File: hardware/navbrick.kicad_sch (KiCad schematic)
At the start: 28 parts, among them J50 Conn_01x06_Pin, J51 Conn_01x06_Pin, SW50 PTS645SK50SMTR92, SW51 PTS645SK50SMTR92, U6 AVR128DA32x-xRXB, U7 FM25L16B

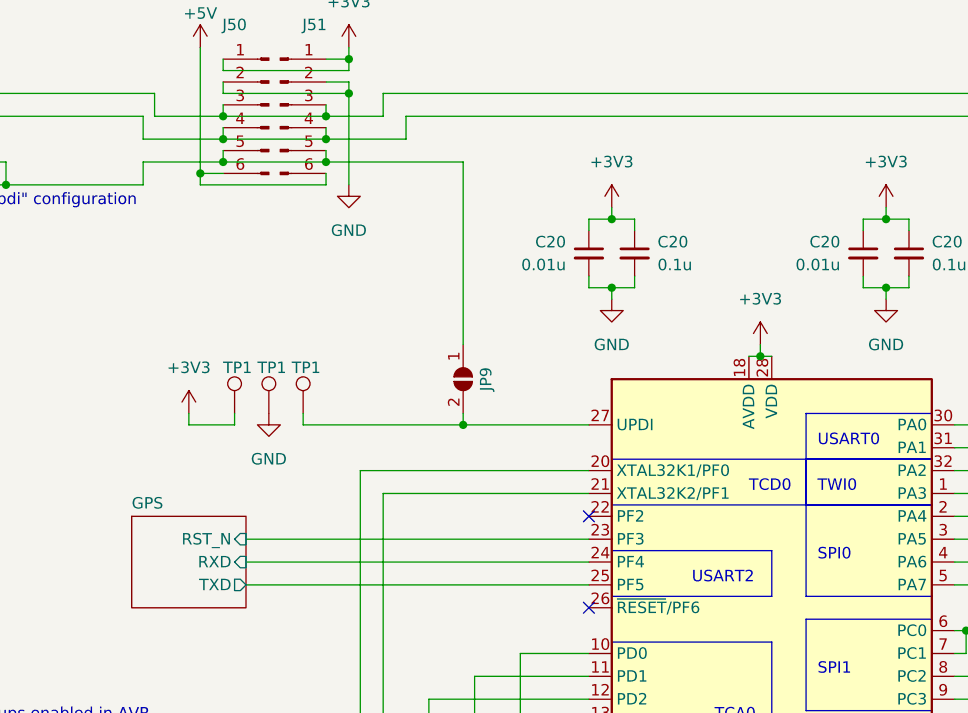
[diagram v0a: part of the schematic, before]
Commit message: Rev B hardware update
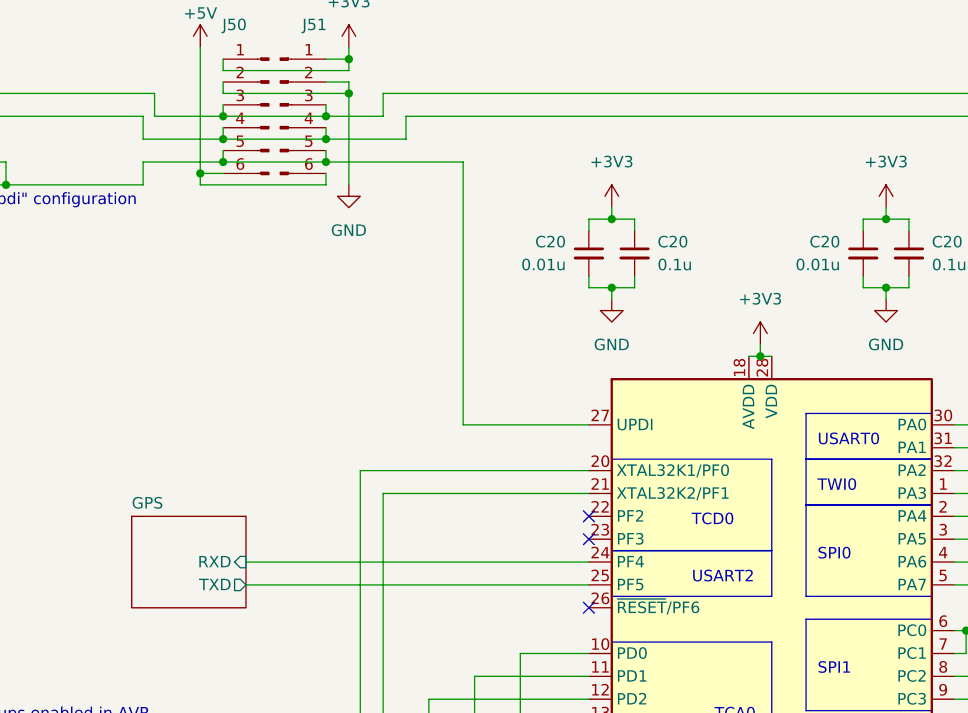
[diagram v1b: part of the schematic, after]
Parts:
- removed JP9: SolderJumper_2_Open, Jumper:SolderJumper-2_P1.3mm_Open_Pad1.0x1.5mm, symbol 0-passives:SolderJumper_2
- removed TP1 (x3): TestPoint, TestPoint:TestPoint_Pad_D2.0mm, symbol Connector:TestPoint
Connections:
- net USB/RxD_1: now also U6.27 (UPDI)
- net GPS/RST_N: no longer names the net of U6.23 (PF3)
- no-connect marks 2 -> 3
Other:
- sheet GPS ports: added none; removed RST_N
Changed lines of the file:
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@@
   (junction (at 53.34 36.83) (diameter 0) (color 0 0 0 0)
-  )
-  (junction (at 104.14 63.5) (diameter 0) (color 0 0 0 0)
   )
   (junction (at 151.13 40.64) (diameter 0) (color 0 0 0 0)
@@
   (no_connect (at 118.11 83.82))
   (no_connect (at 118.11 73.66))
+  (no_connect (at 118.11 76.2))
   (wire (pts (xy 53.34 36.83) (xy 68.58 36.83))
     (stroke (width 0) (type default))
@@
     (stroke (width 0) (type default))
   )
-  (wire (pts (xy 73.66 62.23) (xy 73.66 63.5))
-    (stroke (width 0) (type default))
-  )
   (wire (pts (xy 160.02 86.36) (xy 181.61 86.36))
     (stroke (width 0) (type default))
@@
     (stroke (width 0) (type default))
   )
-  (wire (pts (xy 86.36 62.23) (xy 86.36 63.5))
-    (stroke (width 0) (type default))
-  )
   (wire (pts (xy 92.71 146.05) (xy 92.71 68.58))
     (stroke (width 0) (type default))
@@
     (stroke (width 0) (type default))
   )
-  (wire (pts (xy 104.14 34.29) (xy 104.14 54.61))
+  (wire (pts (xy 104.14 34.29) (xy 104.14 63.5))
     (stroke (width 0) (type default))
   )
@@
     (stroke (width 0) (type default))
   )
-  (wire (pts (xy 104.14 62.23) (xy 104.14 63.5))
-    (stroke (width 0) (type default))
-  )
-  (wire (pts (xy 78.74 63.5) (xy 78.74 62.23))
-    (stroke (width 0) (type default))
-  )
   (wire (pts (xy 53.34 34.29) (xy 52.07 34.29))
     (stroke (width 0) (type default))
@@
     (stroke (width 0) (type default))
   )
-  (wire (pts (xy 86.36 63.5) (xy 104.14 63.5))
-    (stroke (width 0) (type default))
-  )
   (wire (pts (xy 88.9 31.75) (xy 88.9 30.48))
     (stroke (width 0) (type default))
@@
     (stroke (width 0) (type default))
   )
-  (wire (pts (xy 80.01 76.2) (xy 118.11 76.2))
-    (stroke (width 0) (type default))
-  )
   (wire (pts (xy 44.45 113.03) (xy 44.45 115.57))
     (stroke (width 0) (type default))
@@
     (stroke (width 0) (type default))
   )
-  (wire (pts (xy 73.66 63.5) (xy 78.74 63.5))
-    (stroke (width 0) (type default))
-  )
   (rectangle (start 142.24 85.09) (end 156.21 95.25)
     (stroke (width 0) (type default))
     (fill (type none))
   )
-  (rectangle (start 120.65 67.31) (end 142.24 72.39)
+  (rectangle (start 120.65 67.31) (end 138.43 77.47)
     (stroke (width 0) (type default))
     (fill (type none))
@@
     (effects (font (size 1.27 1.27)) (justify left bottom))
   )
-  (text "TCD0" (at 135.89 71.12 0)
+  (text "TCD0" (at 129.54 74.93 0)
     (effects (font (size 1.27 1.27)) (justify left bottom))
   )
@@
         (path "/c26ff3ad-9cdb-4061-8a60-da1ddedb78dd"
           (reference "H53") (unit 1)
-        )
-      )
-    )
-  )
-  (symbol (lib_id "Connector:TestPoint") (at 86.36 62.23 0) (unit 1)
-    (in_bom yes) (on_board yes) (dnp no)
-    (property "Reference" "TP1" (at 85.09 57.15 0)
-      (effects (font (size 1.27 1.27)) (justify left))
-    )
-    (property "Value" "TestPoint" (at 88.9 60.198 0)
-      (effects (font (size 1.27 1.27)) (justify left) hide)
-    )
-    (property "Footprint" "TestPoint:TestPoint_Pad_D2.0mm" (at 91.44 62.23 0)
-      (effects (font (size 1.27 1.27)) hide)
-    )
-    (property "Datasheet" "~" (at 91.44 62.23 0)
-      (effects (font (size 1.27 1.27)) hide)
-    )
-    (pin "1")
-    (instances
-      (project "navbrick"
-        (path "/c26ff3ad-9cdb-4061-8a60-da1ddedb78dd/50a4481b-1e79-4c92-bbac-0068bb0a09ca"
-          (reference "TP1") (unit 1)
-        )
-        (path "/c26ff3ad-9cdb-4061-8a60-da1ddedb78dd"
-          (reference "TP3") (unit 1)
         )
       )
@@
     )
   )
-  (symbol (lib_id "0-power:GND") (at 82.55 62.23 0) (unit 1)
-    (in_bom yes) (on_board yes) (dnp no) (fields_autoplaced)
-    (property "Reference" "#PWR089" (at 82.55 68.58 0)
-      (effects (font (size 1.27 1.27)) hide)
-    )
-    (property "Value" "GND" (at 82.55 67.31 0)
-      (effects (font (size 1.27 1.27)))
-    )
-    (property "Footprint" "" (at 82.55 62.23 0)
-      (effects (font (size 1.27 1.27)) hide)
-    )
-    (property "Datasheet" "" (at 82.55 62.23 0)
-      (effects (font (size 1.27 1.27)) hide)
-    )
-    (pin "1")
-    (instances
-      (project "navbrick"
-        (path "/c26ff3ad-9cdb-4061-8a60-da1ddedb78dd"
-          (reference "#PWR089") (unit 1)
-        )
-      )
-    )
-  )
-  (symbol (lib_id "0-passives:SolderJumper_2") (at 104.14 58.42 270) (unit 1)
-    (in_bom yes) (on_board yes) (dnp no)
-    (property "Reference" "JP9" (at 106.68 58.42 0)
-      (effects (font (size 1.27 1.27)))
-    )
-    (property "Value" "SolderJumper_2_Open" (at 107.95 58.42 0)
-      (effects (font (size 1.27 1.27)) hide)
-    )
-    (property "Footprint" "Jumper:SolderJumper-2_P1.3mm_Open_Pad1.0x1.5mm" (at 104.14 58.42 0)
-      (effects (font (size 1.27 1.27)) hide)
-    )
-    (property "Datasheet" "~" (at 104.14 58.42 0)
-      (effects (font (size 1.27 1.27)) hide)
-    )
-    (pin "1")
-    (pin "2")
-    (instances
-      (project "navbrick"
-        (path "/c26ff3ad-9cdb-4061-8a60-da1ddedb78dd"
-          (reference "JP9") (unit 1)
-        )
-      )
-    )
-  )
   (symbol (lib_id "0-power:+5V") (at 74.93 21.59 0) (unit 1)
     (in_bom yes) (on_board yes) (dnp no) (fields_autoplaced)
@@
     )
   )
-  (symbol (lib_id "0-power:+3V3") (at 73.66 62.23 0) (unit 1)
-    (in_bom yes) (on_board yes) (dnp no) (fields_autoplaced)
-    (property "Reference" "#PWR090" (at 73.66 66.04 0)
-      (effects (font (size 1.27 1.27)) hide)
-    )
-    (property "Value" "+3V3" (at 73.66 57.15 0)
-      (effects (font (size 1.27 1.27)))
-    )
-    (property "Footprint" "" (at 73.66 62.23 0)
-      (effects (font (size 1.27 1.27)) hide)
-    )
-    (property "Datasheet" "" (at 73.66 62.23 0)
-      (effects (font (size 1.27 1.27)) hide)
-    )
-    (pin "1")
-    (instances
-      (project "navbrick"
-        (path "/c26ff3ad-9cdb-4061-8a60-da1ddedb78dd"
-          (reference "#PWR090") (unit 1)
-        )
-      )
-    )
-  )
   (symbol (lib_id "Mechanical:MountingHole") (at 57.15 173.99 0) (unit 1)
     (in_bom yes) (on_board yes) (dnp no) (fields_autoplaced)
@@
     )
   )
-  (symbol (lib_id "Connector:TestPoint") (at 78.74 62.23 0) (unit 1)
-    (in_bom yes) (on_board yes) (dnp no)
-    (property "Reference" "TP1" (at 77.47 57.15 0)
-      (effects (font (size 1.27 1.27)) (justify left))
-    )
-    (property "Value" "TestPoint" (at 81.28 60.198 0)
-      (effects (font (size 1.27 1.27)) (justify left) hide)
-    )
-    (property "Footprint" "TestPoint:TestPoint_Pad_D2.0mm" (at 83.82 62.23 0)
-      (effects (font (size 1.27 1.27)) hide)
-    )
-    (property "Datasheet" "~" (at 83.82 62.23 0)
-      (effects (font (size 1.27 1.27)) hide)
-    )
-    (pin "1")
-    (instances
-      (project "navbrick"
-        (path "/c26ff3ad-9cdb-4061-8a60-da1ddedb78dd/50a4481b-1e79-4c92-bbac-0068bb0a09ca"
-          (reference "TP1") (unit 1)
-        )
-        (path "/c26ff3ad-9cdb-4061-8a60-da1ddedb78dd"
-          (reference "TP2") (unit 1)
-        )
-      )
-    )
-  )
   (symbol (lib_id "Mechanical:MountingHole") (at 76.2 184.15 0) (unit 1)
     (in_bom yes) (on_board yes) (dnp no) (fields_autoplaced)
@@
         (path "/c26ff3ad-9cdb-4061-8a60-da1ddedb78dd"
           (reference "C53") (unit 1)
-        )
-      )
-    )
-  )
-  (symbol (lib_id "Connector:TestPoint") (at 82.55 62.23 0) (unit 1)
-    (in_bom yes) (on_board yes) (dnp no)
-    (property "Reference" "TP1" (at 81.28 57.15 0)
-      (effects (font (size 1.27 1.27)) (justify left))
-    )
-    (property "Value" "TestPoint" (at 85.09 60.198 0)
-      (effects (font (size 1.27 1.27)) (justify left) hide)
-    )
-    (property "Footprint" "TestPoint:TestPoint_Pad_D2.0mm" (at 87.63 62.23 0)
-      (effects (font (size 1.27 1.27)) hide)
-    )
-    (property "Datasheet" "~" (at 87.63 62.23 0)
-      (effects (font (size 1.27 1.27)) hide)
-    )
-    (pin "1")
-    (instances
-      (project "navbrick"
-        (path "/c26ff3ad-9cdb-4061-8a60-da1ddedb78dd/50a4481b-1e79-4c92-bbac-0068bb0a09ca"
-          (reference "TP1") (unit 1)
-        )
-        (path "/c26ff3ad-9cdb-4061-8a60-da1ddedb78dd"
-          (reference "TP4") (unit 1)
         )
       )
@@
       (effects (font (size 1.27 1.27)) (justify right))
     )
-    (pin "RST_N" input (at 80.01 76.2 0)
-      (effects (font (size 1.27 1.27)) (justify right))
-    )
